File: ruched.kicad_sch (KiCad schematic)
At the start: 24 parts, among them J20 USB_C_Receptacle_USB2.0 USB41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, Q6 UMH3N, Q7 DMG2301L, SW1 SW_Push, U1 CP2102N-A02-GQFN24, U6 Heltec_Wireless_shell_V3

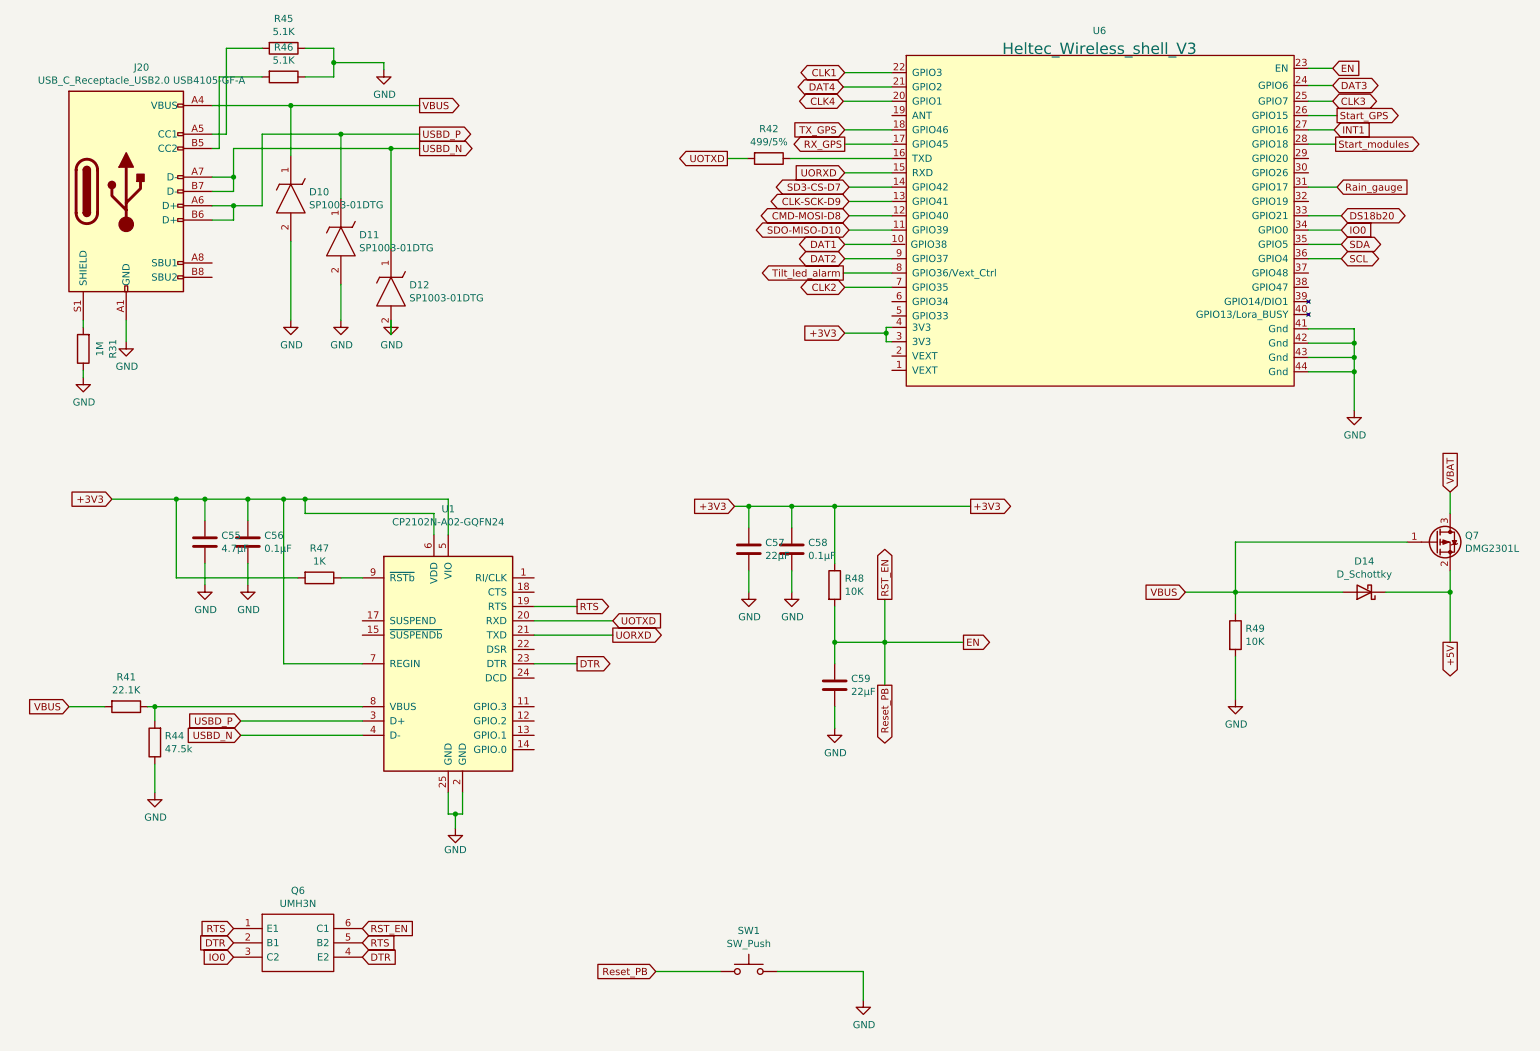
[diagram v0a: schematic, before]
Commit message: Update
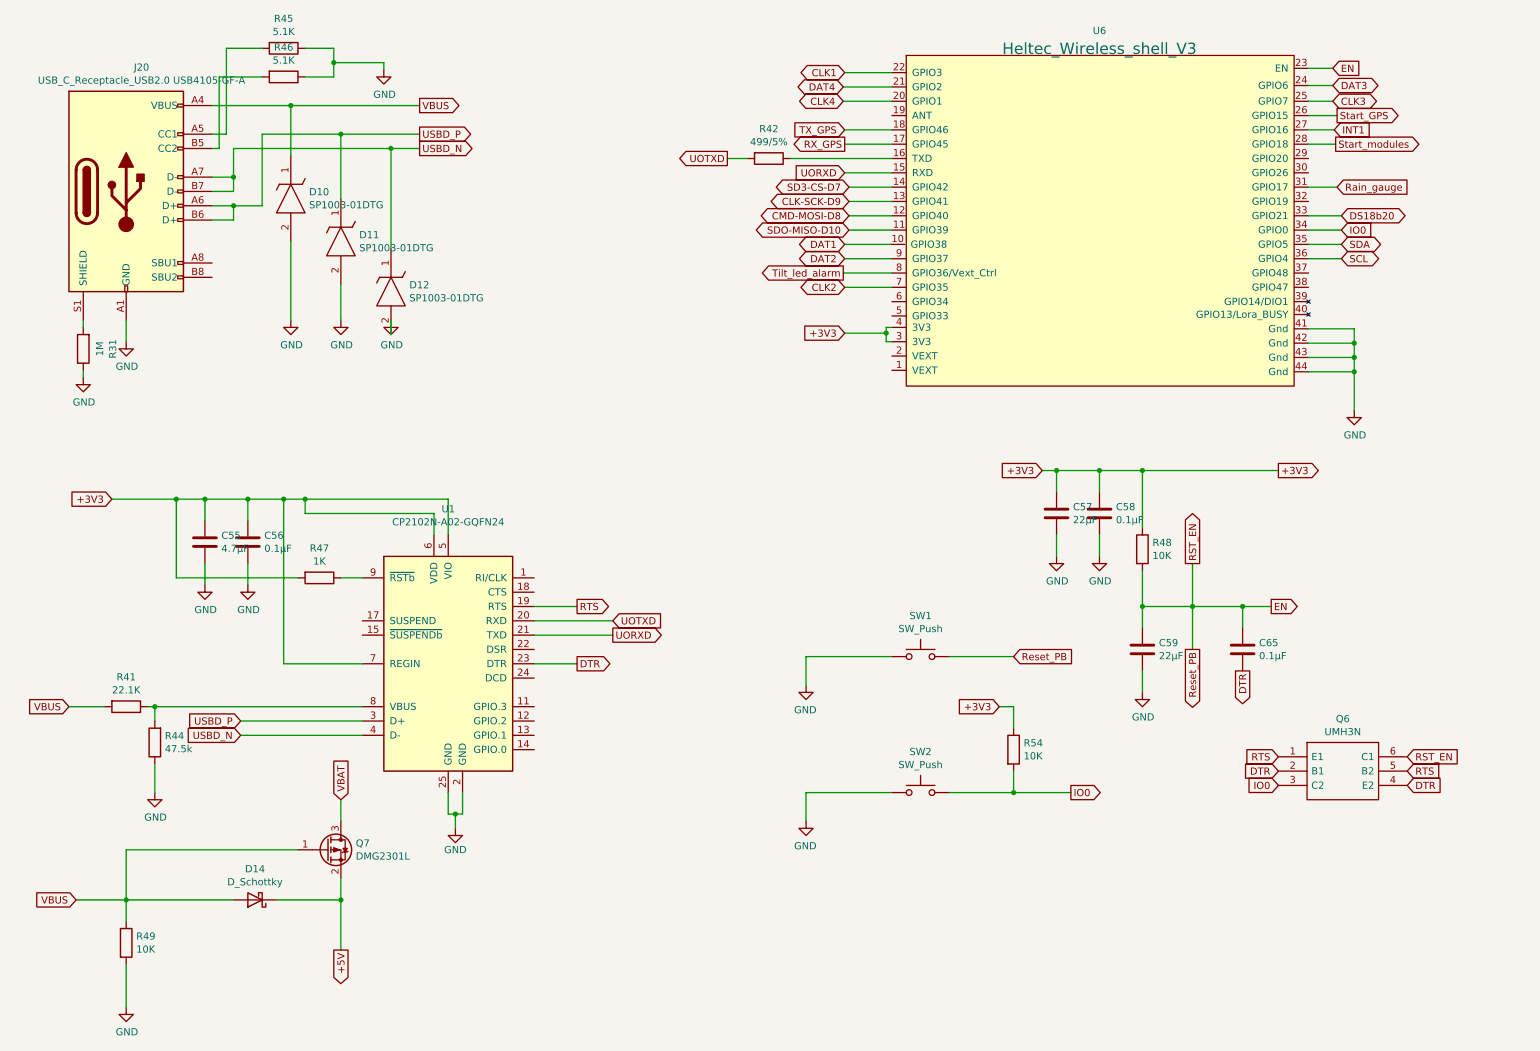
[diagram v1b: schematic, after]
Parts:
- added C65: 0.1µF, Capacitor_SMD:C_0805_2012Metric, symbol Device:C
- added R54: 10K, Resistor_SMD:R_0603_1608Metric, symbol Device:R
- added SW2: SW_Push, Empreintes:PTS636SL43SMTRLFS, symbol Switch:SW_Push
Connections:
- net +3V3: now also R54.1
- net DTR: now also C65.2
- net EN: now also C65.1
- net GND: now also SW2.2
- net IO0: now also R54.2, SW2.1
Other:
- company: (none) -> Ratamuse
- title: (none) -> Open_beehive_scale_board
- moved on the sheet: C57, C58, C59, D14, Q6, Q7, R48, R49, SW1

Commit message: Update
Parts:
- C65: footprint Capacitor_SMD:C_0805_2012Metric -> Capacitor_SMD:C_0603_1608Metric
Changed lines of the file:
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@@
       (effects (font (size 1.27 1.27)) (justify left))
     )
-    (property "Footprint" "Capacitor_SMD:C_0805_2012Metric" (id 2) (at 230.8352 130.81 0)
+    (property "Footprint" "Capacitor_SMD:C_0603_1608Metric" (id 2) (at 230.8352 130.81 0)
       (effects (font (size 1.27 1.27)) hide)
     )

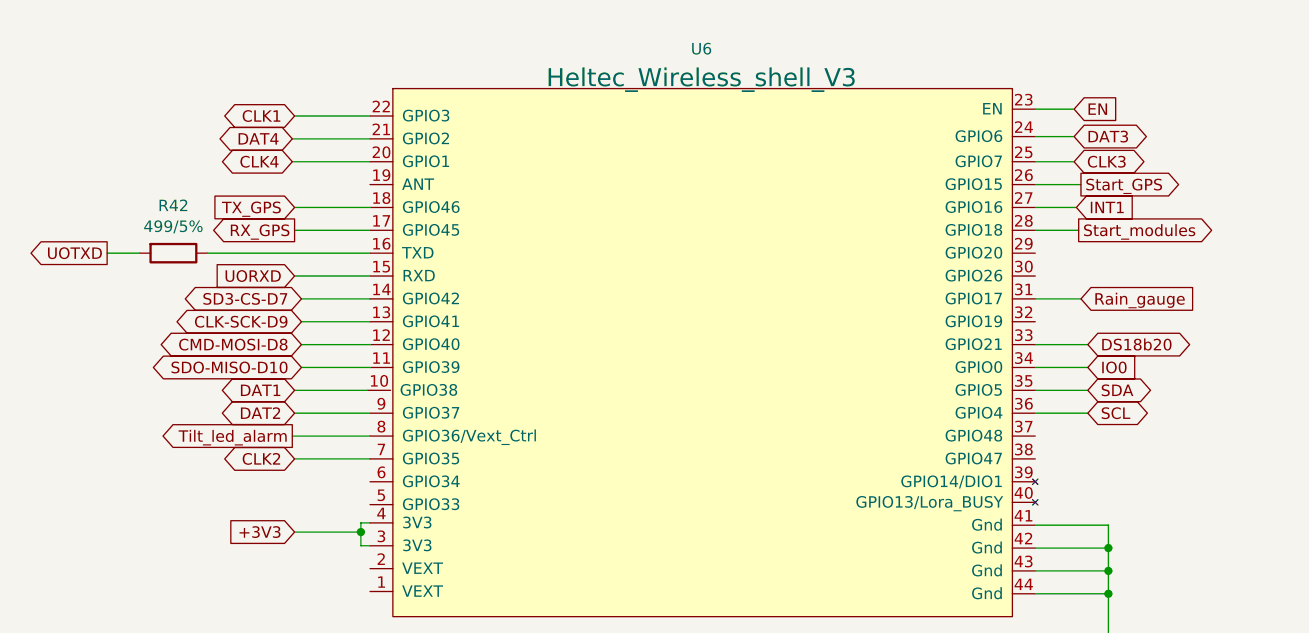
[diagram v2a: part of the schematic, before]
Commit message: Update
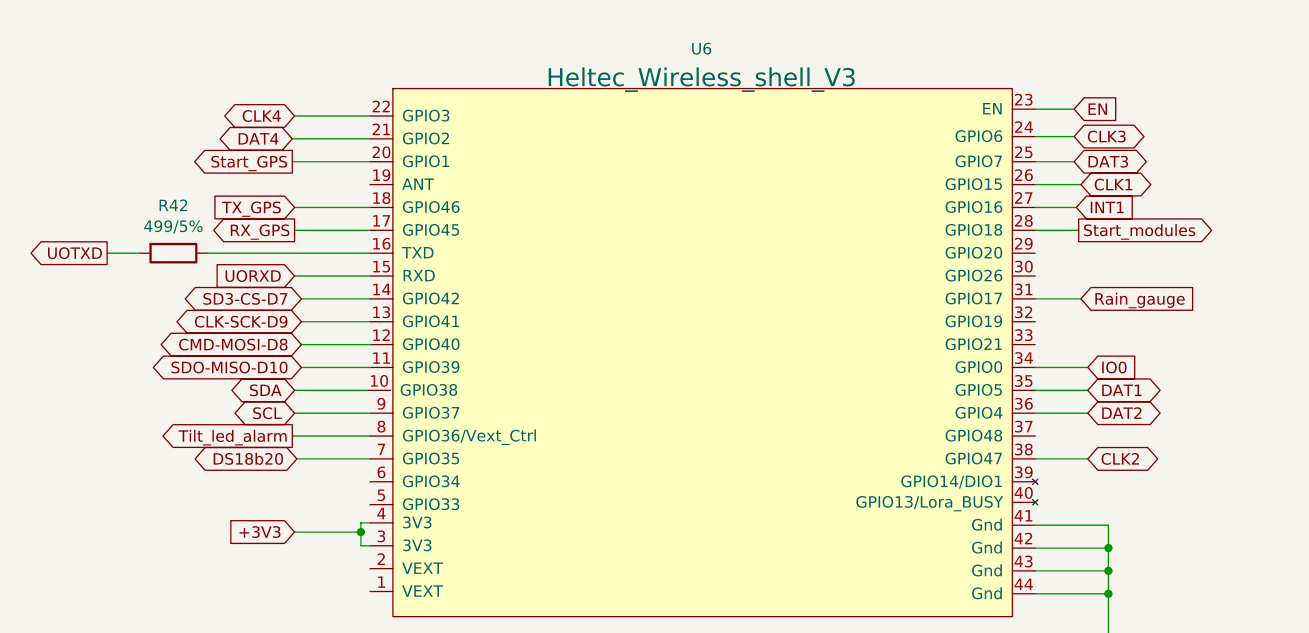
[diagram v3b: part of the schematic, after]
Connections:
- net CLK1: now also U6.26 (GPIO15); no longer U6.22 (GPIO3)
- net CLK2: now also U6.38 (GPIO47); no longer U6.7 (GPIO35)
- net CLK3: now also U6.24 (GPIO6); no longer U6.25 (GPIO7)
- net CLK4: now also U6.22 (GPIO3); no longer U6.20 (GPIO1)
- net DAT1: now also U6.35 (GPIO5); no longer U6.10 (GPIO38)
- net DAT2: now also U6.36 (GPIO4); no longer U6.9 (GPIO37)
- net DAT3: now also U6.25 (GPIO7); no longer U6.24 (GPIO6)
- net DS18b20: now also U6.7 (GPIO35); no longer U6.33 (GPIO21)
- net SCL: now also U6.9 (GPIO37); no longer U6.36 (GPIO4)
- net SDA: now also U6.10 (GPIO38); no longer U6.35 (GPIO5)
- net Start_GPS: now also U6.20 (GPIO1); no longer U6.26 (GPIO15)
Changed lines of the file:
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@@
+    (stroke (width 0) (type default) (color 0 0 0 0))
+  )
+  (wire (pts (xy 241.554 62.738) (xy 247.396 62.738))
     (stroke (width 0) (type default) (color 0 0 0 0))
   )
@@
     (stroke (width 0) (type default) (color 0 0 0 0))
   )
+  (wire (pts (xy 159.512 62.738) (xy 167.64 62.738))
+    (stroke (width 0) (type default) (color 0 0 0 0))
+  )
   (wire (pts (xy 63.5 25.4) (xy 68.58 25.4))
     (stroke (width 0) (type default) (color 0 0 0 0))
@@
     (stroke (width 0) (type default) (color 0 0 0 0))
   )
-  (wire (pts (xy 159.258 62.738) (xy 167.64 62.738))
-    (stroke (width 0) (type default) (color 0 0 0 0))
-  )
   (wire (pts (xy 48.26 38.1) (xy 48.26 25.4))
     (stroke (width 0) (type default) (color 0 0 0 0))
@@
     (stroke (width 0) (type default) (color 0 0 0 0))
   )
-  (wire (pts (xy 241.554 50.038) (xy 247.396 50.038))
-    (stroke (width 0) (type default) (color 0 0 0 0))
-  )
   (wire (pts (xy 86.36 106.68) (xy 86.36 102.87))
     (stroke (width 0) (type default) (color 0 0 0 0))
@@
     )
   )
-  (global_label "CLK3" (shape bidirectional) (at 245.872 29.718 0) (fields_autoplaced)
-    (effects (font (size 1.27 1.27)) (justify left))
-    (property "Intersheet References" "${INTERSHEET_REFS}" (id 0) (at 252.9738 29.6386 0)
+  (global_label "DAT3" (shape bidirectional) (at 245.872 29.718 0) (fields_autoplaced)
+    (effects (font (size 1.27 1.27)) (justify left))
+    (property "Intersheet References" "${INTERSHEET_REFS}" (id 0) (at 252.7319 29.6386 0)
       (effects (font (size 1.27 1.27)) (justify left) hide)
     )
@@
     )
   )
-  (global_label "SDA" (shape bidirectional) (at 247.396 55.118 0) (fields_autoplaced)
-    (effects (font (size 1.27 1.27)) (justify left))
-    (property "Intersheet References" "${INTERSHEET_REFS}" (id 0) (at 253.2883 55.0386 0)
+  (global_label "DAT1" (shape bidirectional) (at 247.396 55.118 0) (fields_autoplaced)
+    (effects (font (size 1.27 1.27)) (justify left))
+    (property "Intersheet References" "${INTERSHEET_REFS}" (id 0) (at 254.2559 55.0386 0)
       (effects (font (size 1.27 1.27)) (justify left) hide)
     )
@@
     )
   )
-  (global_label "CLK2" (shape bidirectional) (at 159.258 62.738 180) (fields_autoplaced)
-    (effects (font (size 1.27 1.27)) (justify right))
-    (property "Intersheet References" "${INTERSHEET_REFS}" (id 0) (at 152.1562 62.6586 0)
-      (effects (font (size 1.27 1.27)) (justify right) hide)
+  (global_label "CLK2" (shape bidirectional) (at 247.396 62.738 0) (fields_autoplaced)
+    (effects (font (size 1.27 1.27)) (justify left))
+    (property "Intersheet References" "${INTERSHEET_REFS}" (id 0) (at 254.4978 62.6586 0)
+      (effects (font (size 1.27 1.27)) (justify left) hide)
     )
   )
@@
     )
   )
-  (global_label "CLK1" (shape bidirectional) (at 159.258 24.638 180) (fields_autoplaced)
+  (global_label "CLK4" (shape bidirectional) (at 159.258 24.638 180) (fields_autoplaced)
     (effects (font (size 1.27 1.27)) (justify right))
     (property "Intersheet References" "${INTERSHEET_REFS}" (id 0) (at 152.1562 24.5586 0)
@@
     )
   )
-  (global_label "Start_GPS" (shape output) (at 246.634 32.258 0) (fields_autoplaced)
-    (effects (font (size 1.27 1.27)) (justify left))
-    (property "Intersheet References" "${INTERSHEET_REFS}" (id 0) (at 258.2715 32.1786 0)
-      (effects (font (size 1.27 1.27)) (justify left) hide)
-    )
-  )
-  (global_label "DAT2" (shape bidirectional) (at 159.258 57.658 180) (fields_autoplaced)
-    (effects (font (size 1.27 1.27)) (justify right))
-    (property "Intersheet References" "${INTERSHEET_REFS}" (id 0) (at 152.3981 57.5786 0)
-      (effects (font (size 1.27 1.27)) (justify right) hide)
-    )
-  )
-  (global_label "SCL" (shape bidirectional) (at 247.396 57.658 0) (fields_autoplaced)
-    (effects (font (size 1.27 1.27)) (justify left))
-    (property "Intersheet References" "${INTERSHEET_REFS}" (id 0) (at 253.2278 57.5786 0)
+  (global_label "CLK1" (shape bidirectional) (at 246.634 32.258 0) (fields_autoplaced)
+    (effects (font (size 1.27 1.27)) (justify left))
+    (property "Intersheet References" "${INTERSHEET_REFS}" (id 0) (at 253.7358 32.1786 0)
+      (effects (font (size 1.27 1.27)) (justify left) hide)
+    )
+  )
+  (global_label "SCL" (shape bidirectional) (at 159.258 57.658 180) (fields_autoplaced)
+    (effects (font (size 1.27 1.27)) (justify right))
+    (property "Intersheet References" "${INTERSHEET_REFS}" (id 0) (at 153.4262 57.5786 0)
+      (effects (font (size 1.27 1.27)) (justify right) hide)
+    )
+  )
+  (global_label "DAT2" (shape bidirectional) (at 247.396 57.658 0) (fields_autoplaced)
+    (effects (font (size 1.27 1.27)) (justify left))
+    (property "Intersheet References" "${INTERSHEET_REFS}" (id 0) (at 254.2559 57.5786 0)
       (effects (font (size 1.27 1.27)) (justify left) hide)
     )
@@
     )
   )
-  (global_label "DAT3" (shape bidirectional) (at 245.872 26.924 0) (fields_autoplaced)
-    (effects (font (size 1.27 1.27)) (justify left))
-    (property "Intersheet References" "${INTERSHEET_REFS}" (id 0) (at 252.7319 26.8446 0)
+  (global_label "CLK3" (shape bidirectional) (at 245.872 26.924 0) (fields_autoplaced)
+    (effects (font (size 1.27 1.27)) (justify left))
+    (property "Intersheet References" "${INTERSHEET_REFS}" (id 0) (at 252.9738 26.8446 0)
       (effects (font (size 1.27 1.27)) (justify left) hide)
     )
@@
     )
   )
-  (global_label "DS18b20" (shape bidirectional) (at 247.396 50.038 0) (fields_autoplaced)
-    (effects (font (size 1.27 1.27)) (justify left))
-    (property "Intersheet References" "${INTERSHEET_REFS}" (id 0) (at 258.1869 49.9586 0)
-      (effects (font (size 1.27 1.27)) (justify left) hide)
+  (global_label "DS18b20" (shape bidirectional) (at 159.512 62.738 180) (fields_autoplaced)
+    (effects (font (size 1.27 1.27)) (justify right))
+    (property "Intersheet References" "${INTERSHEET_REFS}" (id 0) (at 148.7211 62.6586 0)
+      (effects (font (size 1.27 1.27)) (justify right) hide)
     )
   )
@@
     )
   )
-  (global_label "DAT1" (shape bidirectional) (at 159.258 55.118 180) (fields_autoplaced)
-    (effects (font (size 1.27 1.27)) (justify right))
-    (property "Intersheet References" "${INTERSHEET_REFS}" (id 0) (at 152.3981 55.0386 0)
+  (global_label "SDA" (shape bidirectional) (at 159.258 55.118 180) (fields_autoplaced)
+    (effects (font (size 1.27 1.27)) (justify right))
+    (property "Intersheet References" "${INTERSHEET_REFS}" (id 0) (at 153.3657 55.0386 0)
       (effects (font (size 1.27 1.27)) (justify right) hide)
     )
@@
     )
   )
-  (global_label "CLK4" (shape bidirectional) (at 159.004 29.718 180) (fields_autoplaced)
-    (effects (font (size 1.27 1.27)) (justify right))
-    (property "Intersheet References" "${INTERSHEET_REFS}" (id 0) (at 151.9022 29.6386 0)
-      (effects (font (size 1.27 1.27)) (justify right) hide)
-    )
+  (global_label "Start_GPS" (shape output) (at 159.004 29.718 180) (fields_autoplaced)
+    (effects (font (size 1.27 1.27)) (justify right))
+    (property "Intersheet References" "${INTERSHEET_REFS}" (id 0) (at 147.3665 29.6386 0)
+      (effects (font (size 1.27 1.27)) (justify right) hide)
+    )

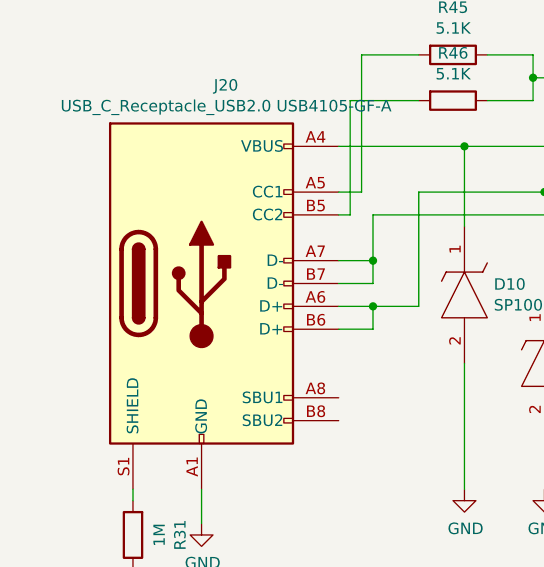
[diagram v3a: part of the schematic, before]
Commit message: update
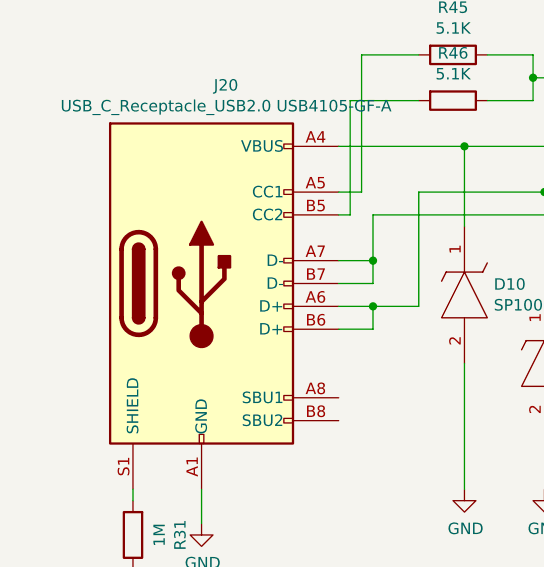
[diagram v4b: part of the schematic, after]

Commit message: Revert "update"
This reverts commit 9afc669c055c7e8087787cb6fdf10dddd7845243.
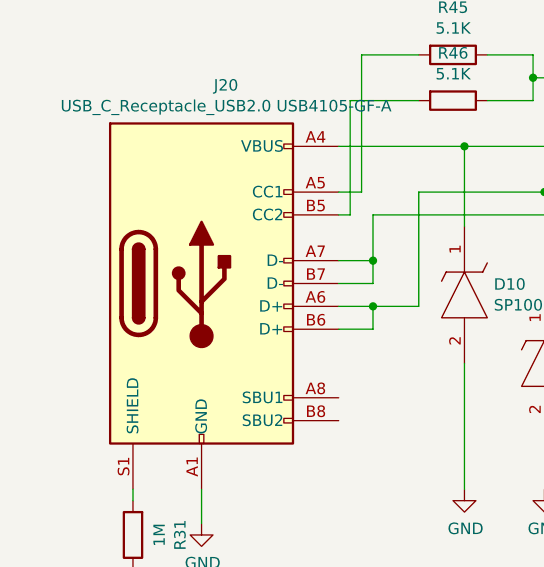
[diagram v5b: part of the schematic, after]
